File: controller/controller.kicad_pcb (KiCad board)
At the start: 2 copper layers, 9 parts, among them U1 Joystick

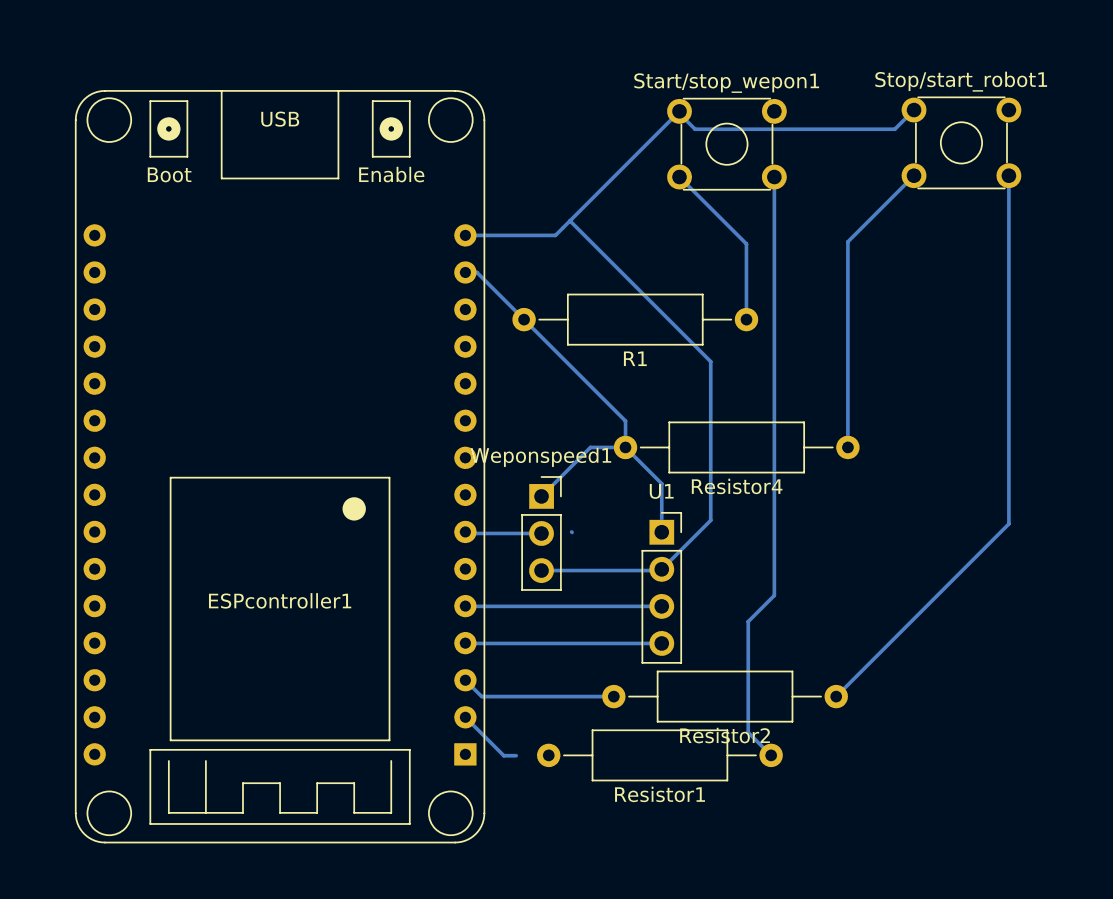
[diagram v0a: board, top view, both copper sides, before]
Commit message: added the pcb design for the controller
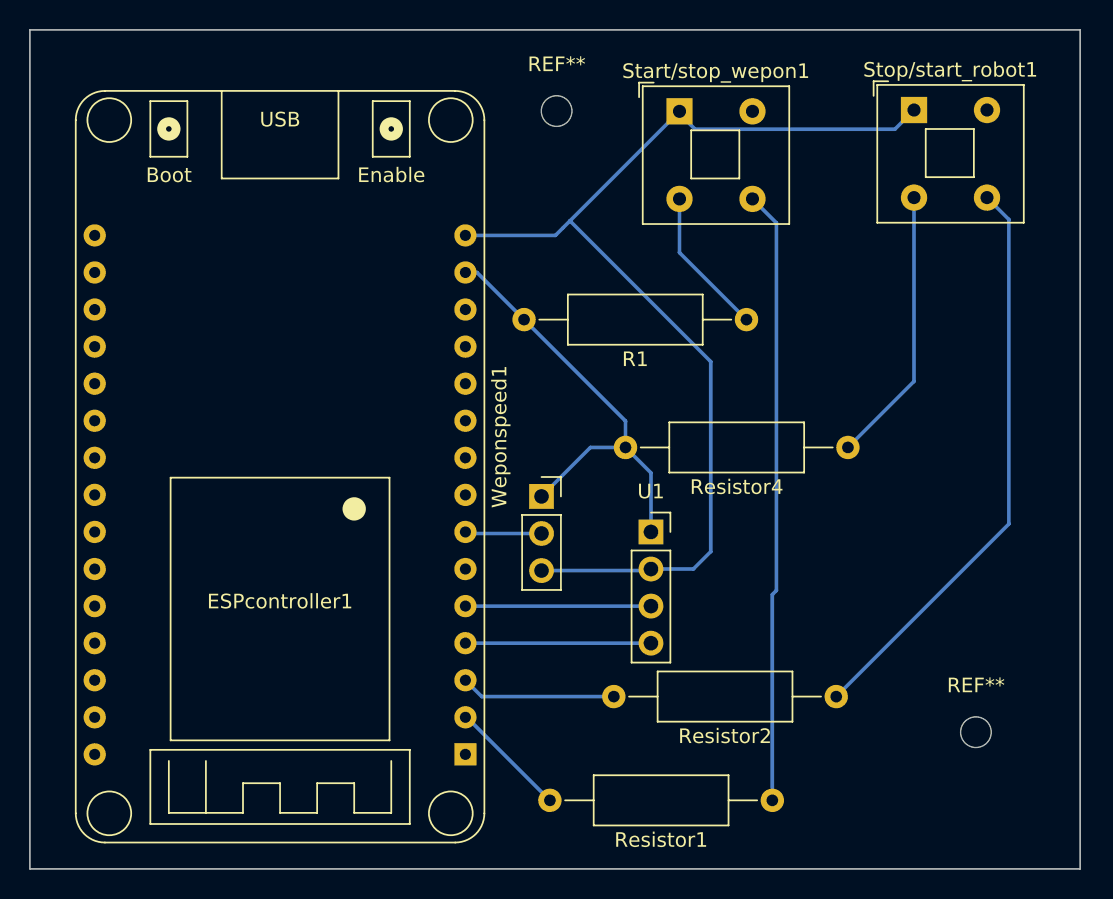
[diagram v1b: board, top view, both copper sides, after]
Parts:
- added REF**: MountingHole_2.1mm, MountingHole:MountingHole_2.1mm, F.Cu at (112.9, 75.3)
- added REF**: MountingHole_2.1mm, MountingHole:MountingHole_2.1mm, F.Cu at (141.7, 117.9)
- Start/stop_wepon1: footprint Button_Switch_THT:SW_TH_Tactile_Omron_B3F-10xx -> Button_Switch_THT:SW_Push_2P1T_Toggle_CK_PVA1xxH4xxxxxxV2
- Stop/start_robot1: footprint Button_Switch_THT:SW_TH_Tactile_Omron_B3F-10xx -> Button_Switch_THT:SW_Push_2P1T_Toggle_CK_PVA1xxH3xxxxxxV2
- moved Resistor1 3.08 mm to (127.7, 122.5)
- moved U1 0.74 mm to (119.4, 104.1)
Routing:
- net Net-(ESPcontroller1-Pad2): track 4.57 -> 8.15 mm
- net Net-(Resistor4-Pad1): track 20.6 -> 19.0 mm
- net Net-(R1-Pad1): track 11.7 -> 10.2 mm
- net Net-(Resistor1-Pad1): track 41.0 -> 42.0 mm
- net Net-(ESPcontroller1-Pad15): track 73.1 -> 74.0 mm
- net Net-(Resistor2-Pad1): track 40.6 -> 39.7 mm
- net Net-(ESPcontroller1-Pad5): track 13.5 -> 12.7 mm
- net Net-(ESPcontroller1-Pad4): track 13.5 -> 12.7 mm
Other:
- board outline added: 72 x 57.5 mm
